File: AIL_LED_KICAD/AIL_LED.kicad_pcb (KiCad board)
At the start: 2 copper layers, 40 x 22 mm, 22 parts, among them J1 Conn_01x02_Female

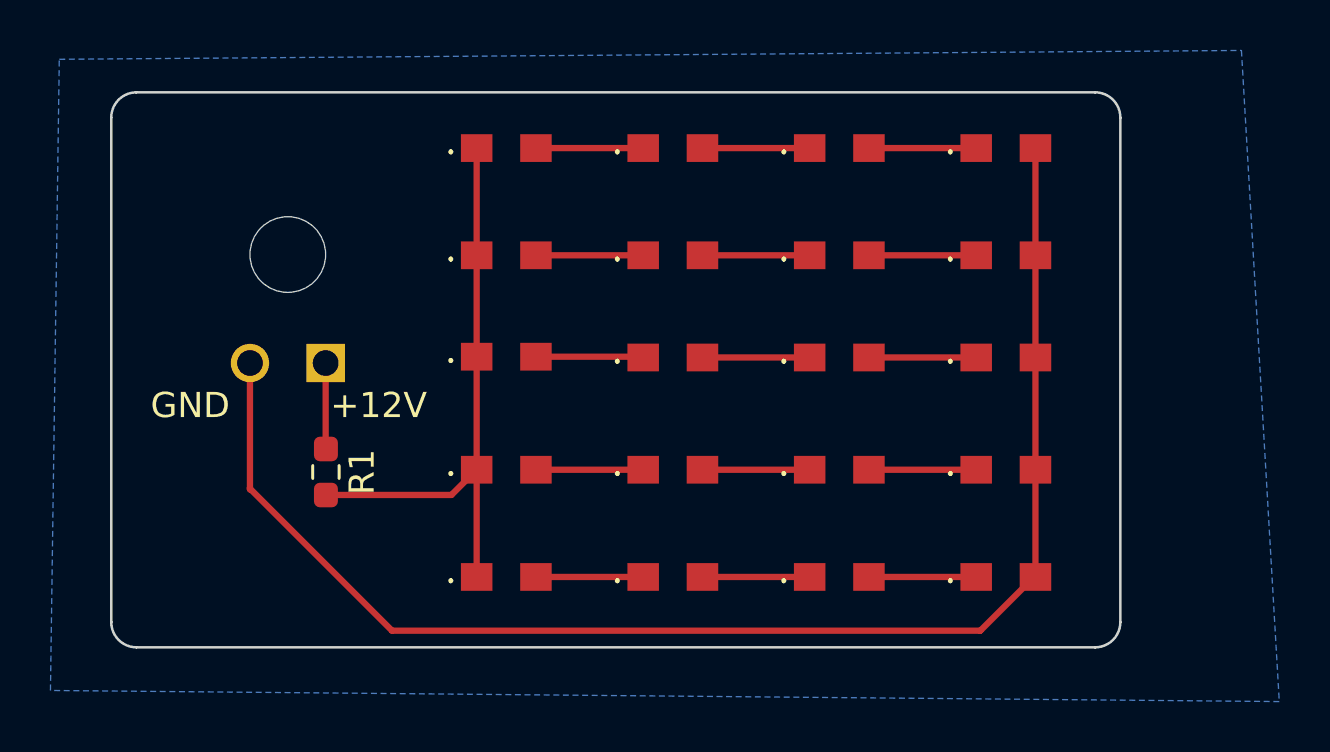
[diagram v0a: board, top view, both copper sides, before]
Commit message: updating with BOM
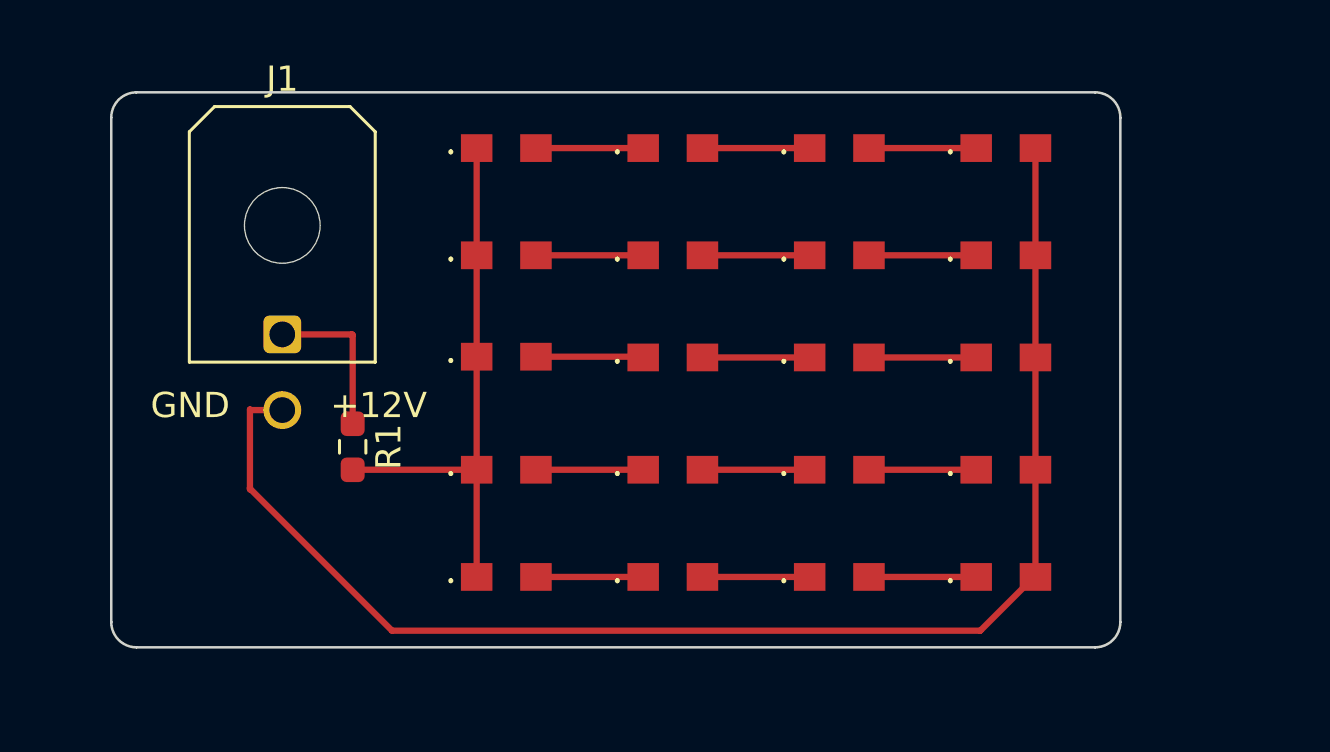
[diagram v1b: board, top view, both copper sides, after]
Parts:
- J1: footprint Connector 215760-1002:215760-YY02 -> Connector_Molex:Molex_Micro-Fit_3.0_43045-0200_2x01_P3.00mm_Horizontal; moved to F.Cu
- moved J1 2.06 mm to (176.8, 97.6)
- moved R1 1.46 mm to (179.6, 102.0)
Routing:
- net +12V: track 3.41 -> 6.32 mm
- net Net-(LED1-Pad1): track 23.4 -> 21.9 mm
- net GND: track 56.4 -> 55.8 mm
- removed copper zone on B.Cu, net GND
